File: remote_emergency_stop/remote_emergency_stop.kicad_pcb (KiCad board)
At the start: 2 copper layers, 1 part, among them U1 MOUDLE-SEEEDUINO-XIAO-ESP32C3

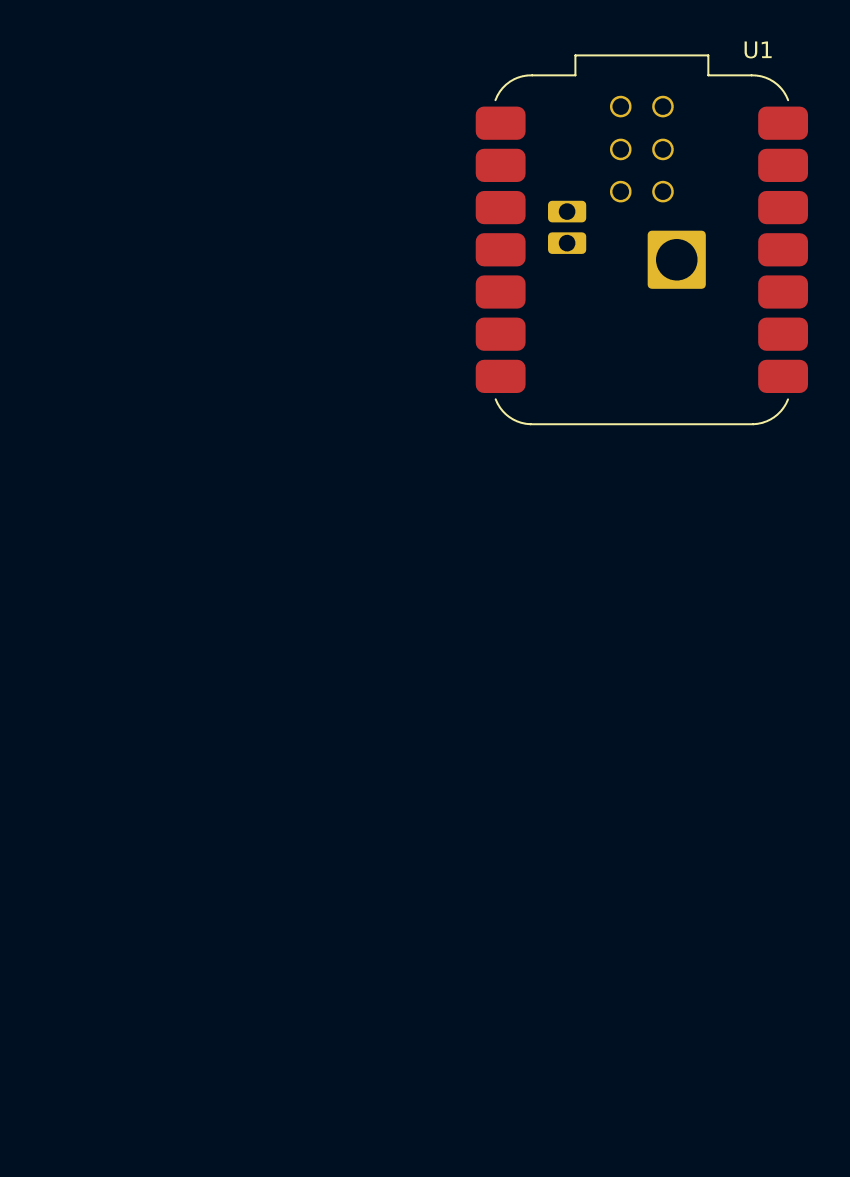
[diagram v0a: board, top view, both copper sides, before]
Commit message: こりゃだめだ、ユーザーインタフェイスが整ってない。
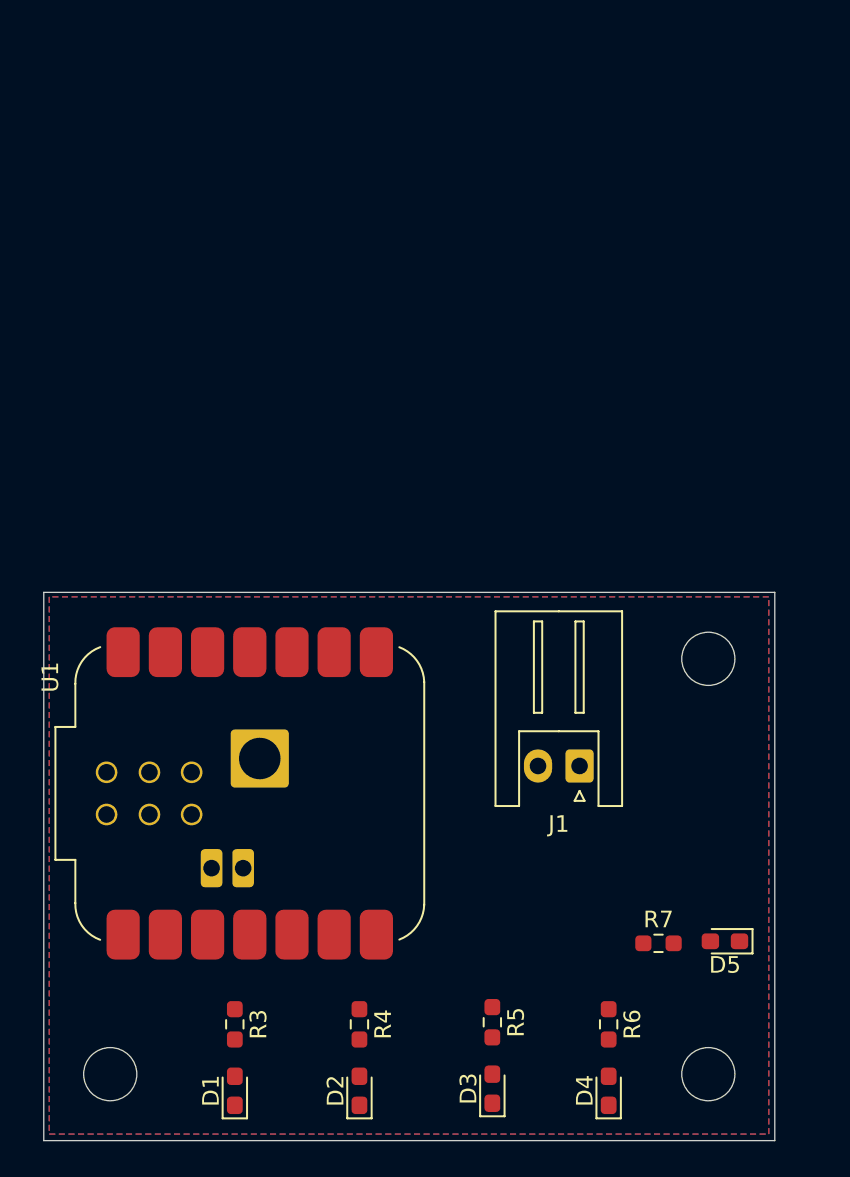
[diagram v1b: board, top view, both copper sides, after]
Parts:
- added D1: LED, LED_SMD:LED_0603_1608Metric_Pad1.05x0.95mm_HandSolder, F.Cu at (127.5, 147.0)
- added D2: LED, LED_SMD:LED_0603_1608Metric_Pad1.05x0.95mm_HandSolder, F.Cu at (135.0, 147.0)
- added D3: LED, LED_SMD:LED_0603_1608Metric_Pad1.05x0.95mm_HandSolder, F.Cu at (143.0, 146.9)
- added D4: LED, LED_SMD:LED_0603_1608Metric_Pad1.05x0.95mm_HandSolder, F.Cu at (150.0, 147.0)
- added D5: LED, LED_SMD:LED_0603_1608Metric_Pad1.05x0.95mm_HandSolder, F.Cu at (157.0, 138.0)
- added J1: Conn_01x02, Connector_JST:JST_XH_S2B-XH-A_1x02_P2.50mm_Horizontal, F.Cu at (148.2, 127.5)
- added R3: 1K, Resistor_SMD:R_0603_1608Metric_Pad0.98x0.95mm_HandSolder, F.Cu at (127.5, 143.0)
- added R4: 1K, Resistor_SMD:R_0603_1608Metric_Pad0.98x0.95mm_HandSolder, F.Cu at (135.0, 143.0)
- added R5: 1K, Resistor_SMD:R_0603_1608Metric_Pad0.98x0.95mm_HandSolder, F.Cu at (143.0, 142.9)
- added R6: 1K, Resistor_SMD:R_0603_1608Metric_Pad0.98x0.95mm_HandSolder, F.Cu at (150.0, 143.0)
- added R7: 500, Resistor_SMD:R_0603_1608Metric_Pad0.98x0.95mm_HandSolder, F.Cu at (153.0, 138.1)
- added REF**: MountingHole_3.2mm_M3, MountingHole:MountingHole_3.2mm_M3, F.Cu at (120.0, 146.0)
- added REF**: MountingHole_3.2mm_M3, MountingHole:MountingHole_3.2mm_M3, F.Cu at (156.0, 121.0)
- added REF**: MountingHole_3.2mm_M3, MountingHole:MountingHole_3.2mm_M3, F.Cu at (156.0, 146.0)
- moved U1 40.3 mm to (128.4, 129.1), turned to 90 degrees
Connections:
- U1 pad 1: unconnected-(U1-PA02_A0_D0-Pad1) -> LED1
- U1 pad 11: unconnected-(U1-PA6_A10_D10_MOSI-Pad11) -> ENABLE
- U1 pad 12: unconnected-(U1-3V3-Pad12) -> +3.3V
- U1 pad 13: unconnected-(U1-GND-Pad13) -> GND
- U1 pad 14: unconnected-(U1-5V-Pad14) -> +5V
- U1 pad 2: unconnected-(U1-PA4_A1_D1-Pad2) -> LED2
- U1 pad 3: unconnected-(U1-PA10_A2_D2-Pad3) -> LED3
- U1 pad 4: unconnected-(U1-PA11_A3_D3-Pad4) -> LED4
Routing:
- added copper zone on B.Cu, net GND
- added copper zone on F.Cu, net GND
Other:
- board outline added: 44 x 33 mm

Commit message: 遠隔非常停止は回路だけ完成した気がする
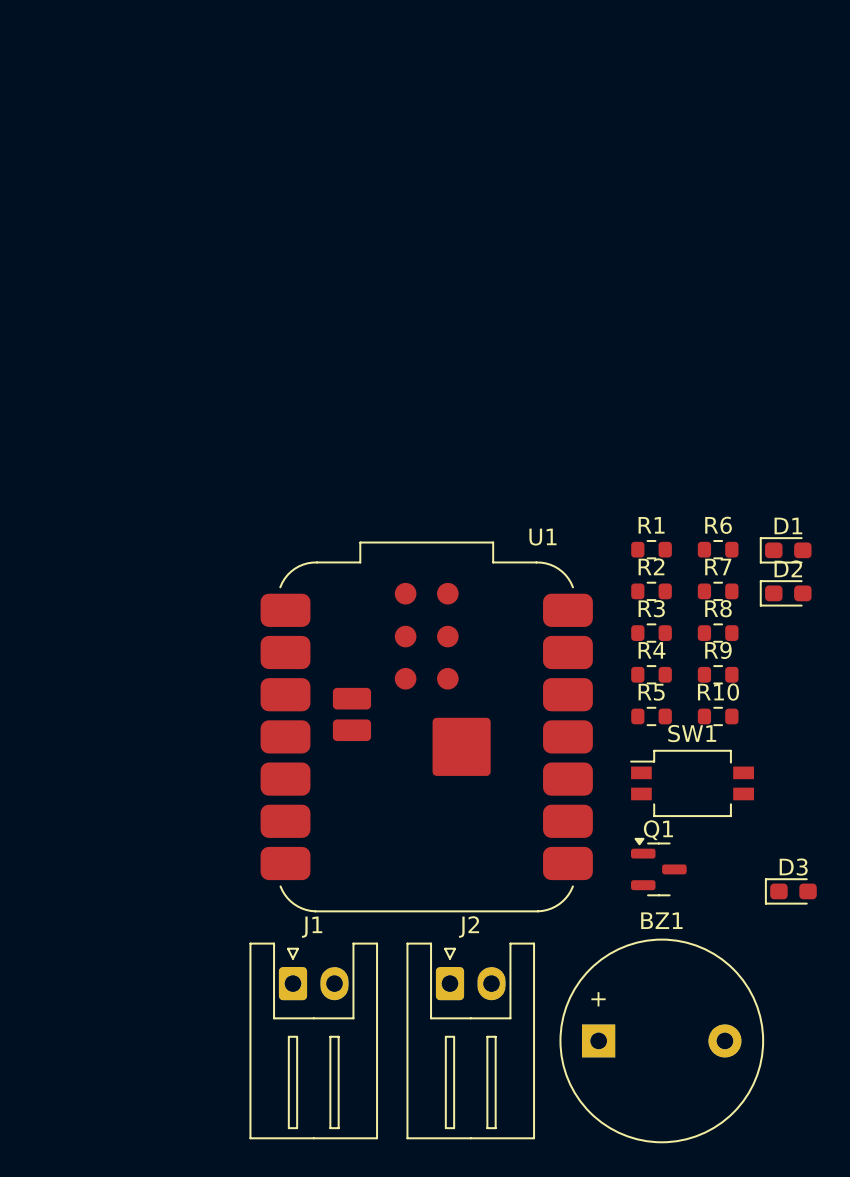
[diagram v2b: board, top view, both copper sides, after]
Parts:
- removed D4, D5: LED, LED_SMD:LED_0603_1608Metric_Pad1.05x0.95mm_HandSolder
- removed REF** (x3): MountingHole_3.2mm_M3, MountingHole:MountingHole_3.2mm_M3
- added BZ1: Buzzer, Buzzer_Beeper:Buzzer_12x9.5RM7.6, F.Cu at (149.4, 144.0)
- added J2: Conn_01x02, Connector_JST:JST_XH_S2B-XH-A_1x02_P2.50mm_Horizontal, F.Cu at (140.4, 140.6)
- added Q1: BSS138, Package_TO_SOT_SMD:SOT-23, F.Cu at (153.0, 133.7)
- added R1: 220K, Resistor_SMD:R_0603_1608Metric, F.Cu at (152.6, 114.4)
- added R10: 1K, Resistor_SMD:R_0603_1608Metric, F.Cu at (156.6, 124.5)
- added R2: 220K, Resistor_SMD:R_0603_1608Metric, F.Cu at (152.6, 116.9)
- added R8: 500, Resistor_SMD:R_0603_1608Metric, F.Cu at (156.6, 119.5)
- added R9: 1K, Resistor_SMD:R_0603_1608Metric, F.Cu at (156.6, 122.0)
- added SW1: SW_DIP_x02, Button_Switch_SMD:SW_DIP_SPSTx02_Slide_Omron_A6H-2101_W6.15mm_P1.27mm, F.Cu at (155.1, 128.5)
- D1: value LED -> Yellow
- D2: value LED -> Blue
- D3: value LED -> Red
- R3, R4, R5: value 1K -> 10K; footprint Resistor_SMD:R_0603_1608Metric_Pad0.98x0.95mm_HandSolder -> Resistor_SMD:R_0603_1608Metric
- R6: footprint Resistor_SMD:R_0603_1608Metric_Pad0.98x0.95mm_HandSolder -> Resistor_SMD:R_0603_1608Metric
- R7: value 500 -> 20K; footprint Resistor_SMD:R_0603_1608Metric_Pad0.98x0.95mm_HandSolder -> Resistor_SMD:R_0603_1608Metric
- moved D1 46.6 mm to (160.8, 114.5), turned to 0 degrees
- moved D2 39.5 mm to (160.8, 117.1), turned to 0 degrees
- moved R3 34.4 mm to (152.6, 119.5), turned to 0 degrees
- moved R6 29.3 mm to (156.6, 114.4), turned to 0 degrees
- moved R4 27.4 mm to (152.6, 122.0), turned to 0 degrees
- moved D3 21.7 mm to (161.1, 135.0), turned to 0 degrees
- moved J1 21.7 mm to (131.0, 140.6), turned to 0 degrees
- moved R7 21.5 mm to (156.6, 116.9)
- moved R5 20.7 mm to (152.6, 124.5), turned to 0 degrees
- moved U1 11.2 mm to (139.1, 125.7), turned to 0 degrees
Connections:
- D1 pad 1: GND -> Net-(BZ1--)
- R3 pad 1: LED1 -> DIP1
- R3 pad 2: Net-(D1-A) -> GND
- R4 pad 1: LED2 -> DIP2
- R4 pad 2: Net-(D2-A) -> GND
- R5 pad 1: LED3 -> GND
- R5 pad 2: Net-(D3-A) -> SW
- R6 pad 1: LED4 -> ENABLE
- R6 pad 2: Net-(D4-A) -> Net-(Q1-G)
- R7 pad 1: ENABLE -> Net-(Q1-G)
- R7 pad 2: Net-(D5-A) -> GND
- U1 pad 1: LED1 -> BAT_LEVEL
- U1 pad 11: ENABLE -> unconnected-(U1-PA6_A10_D10_MOSI-Pad11)
- U1 pad 2: LED2 -> WIRELESS
- U1 pad 3: LED3 -> ENABLE
- U1 pad 4: LED4 -> DIP1
- U1 pad 5: unconnected-(U1-PA8_A4_D4_SDA-Pad5) -> DIP2
- U1 pad 6: unconnected-(U1-PA9_A5_D5_SCL-Pad6) -> SW
- U1 pad 8: unconnected-(U1-PB09_A7_D7_RX-Pad8) -> BAT_LOW
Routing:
- removed copper zone on B.Cu, net GND
- removed copper zone on F.Cu, net GND
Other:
- board outline removed
